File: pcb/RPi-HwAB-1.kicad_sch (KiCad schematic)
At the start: 5 parts, among them U1 CAT24C256

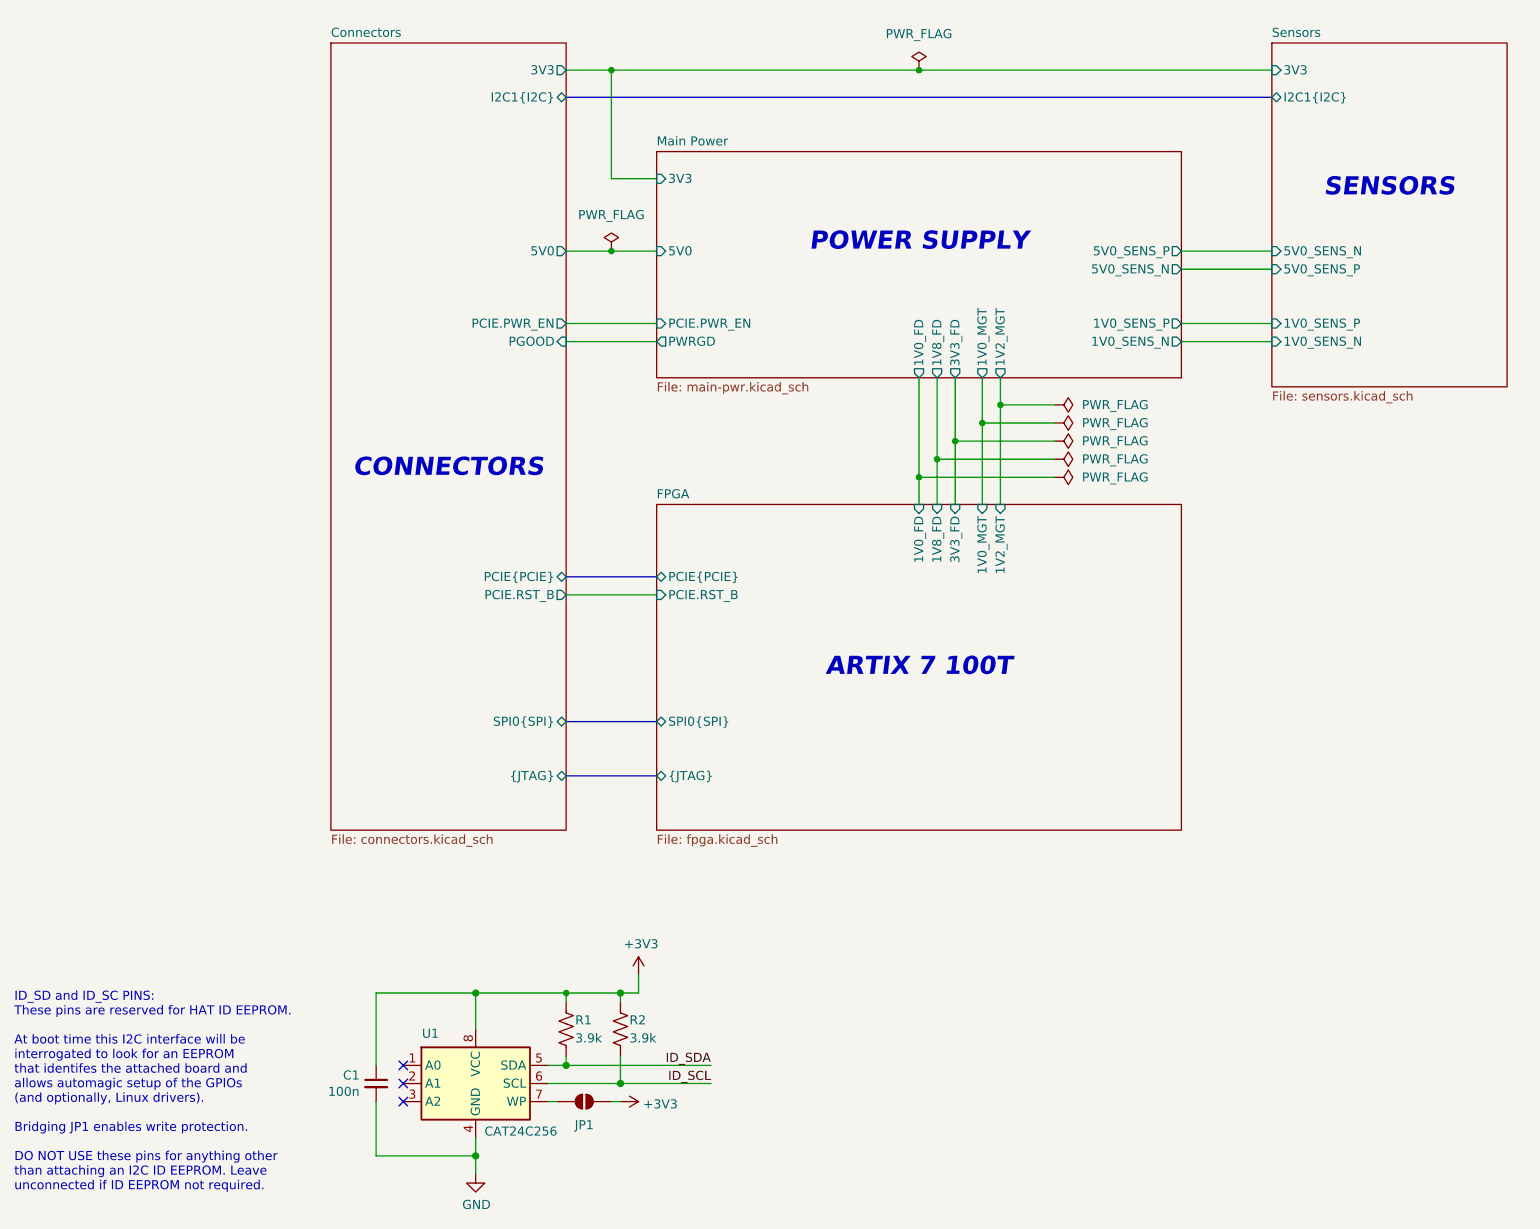
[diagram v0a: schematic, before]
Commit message: power restructuring
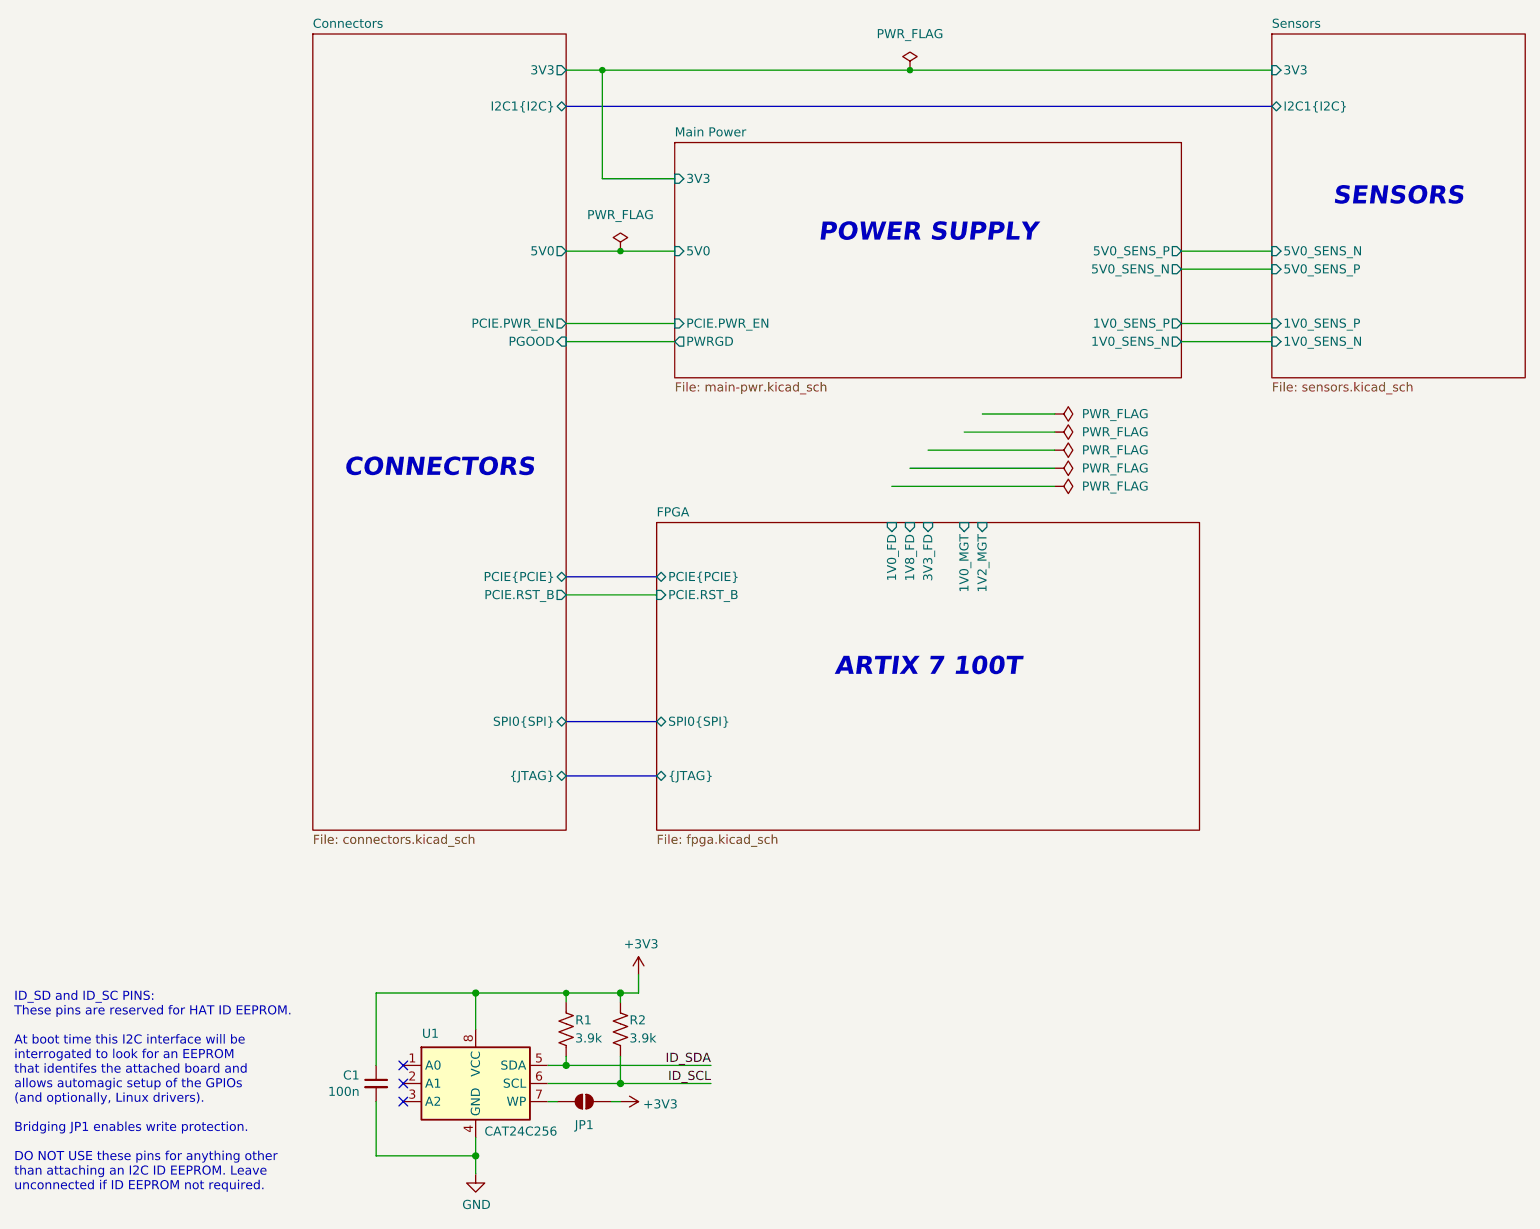
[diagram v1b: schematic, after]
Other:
- sheet Main Power ports: added none; removed 1V0_FD, 1V0_MGT, 1V2_MGT, 1V8_FD, 3V3_FD
